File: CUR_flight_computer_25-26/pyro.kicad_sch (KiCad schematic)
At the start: 22 parts, among them J2 PYRO, J3 PYRO, J4 PYRO, J5 PYRO, U4 BUK9K25-40RAX, U5 BUK9K25-40RAX

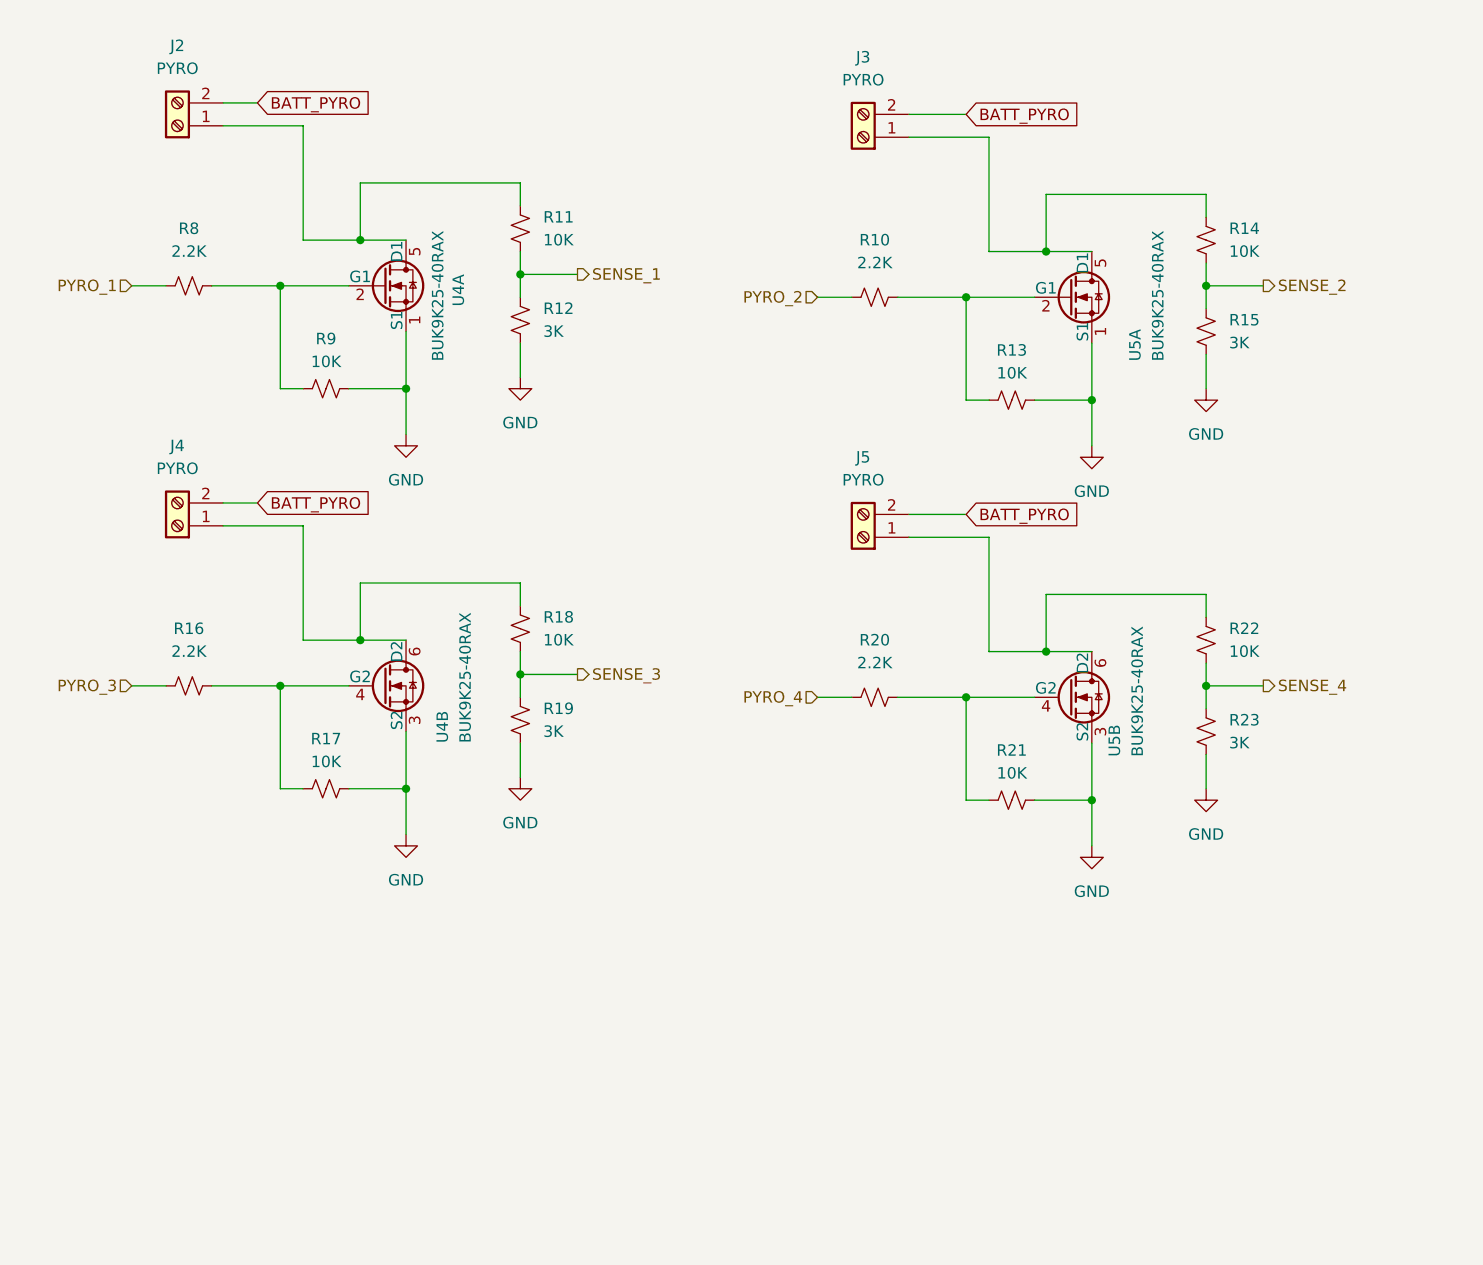
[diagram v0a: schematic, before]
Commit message: added dubugging
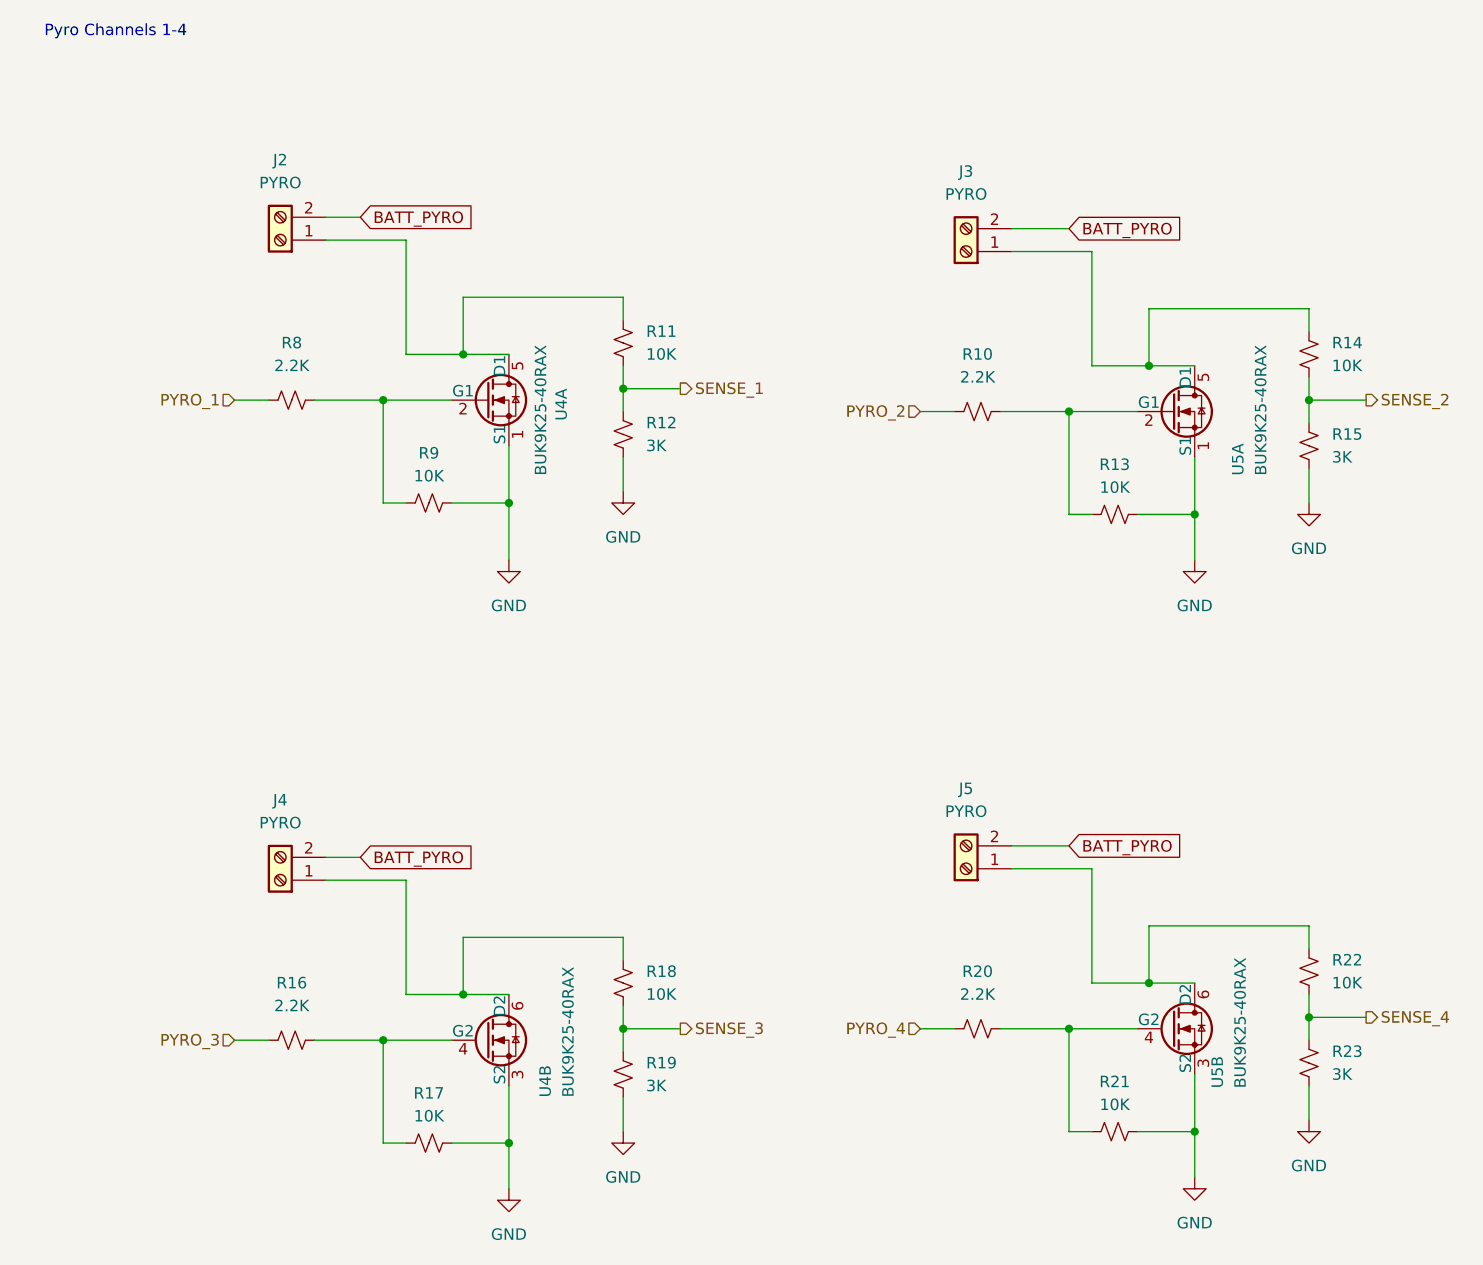
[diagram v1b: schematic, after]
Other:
- note added: "Pyro Channels 1-4"
- moved on the sheet: J2, J3, J4, J5, R10, R11, R12, R13, R14, R15, R16, R17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
